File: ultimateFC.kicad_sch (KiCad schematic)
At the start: 205 parts, among them J1 USB_B_Micro, U1 LMR33630CQRNX, U2 TPS62824ADMQ, U3 LMR33620CRNXT, U4 S25FL064L, U5 DPS310, U6 BMI270, U7 STM32H735VGH6, U8 ICM-20602, Y1 CSTNE8M00G550000R0

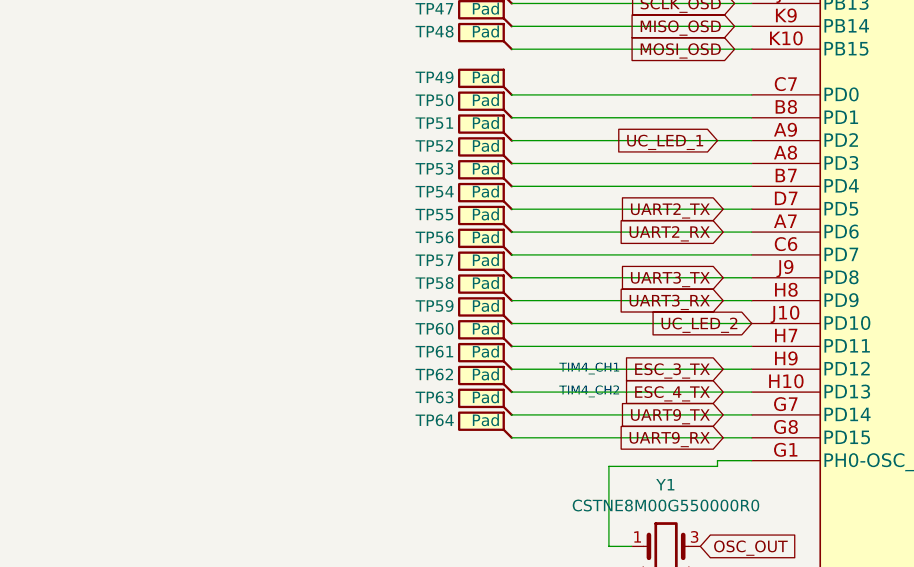
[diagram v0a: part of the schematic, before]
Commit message: more layout
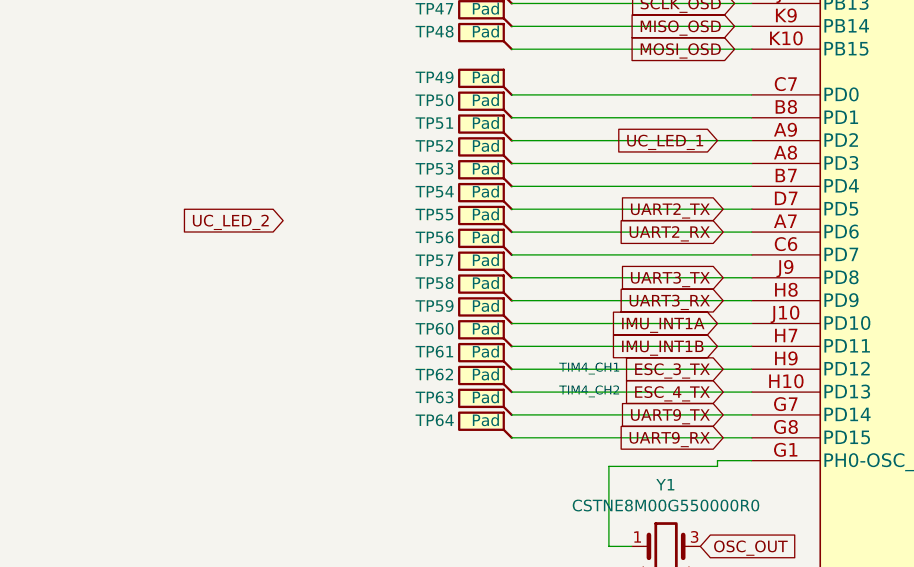
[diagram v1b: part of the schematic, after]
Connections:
- net UC_LED_2: no longer TP59.1, U7.J10 (PD10)
- net IMU_INT1B: now reaches TP60.1, U7.H7 (PD11)
- new net IMU_INT1A: TP59.1, U7.J10 (PD10)
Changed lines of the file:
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@@
+    )
+  )
+  (global_label "IMU_INT1A" (shape input) (at 538.48 127 180) (fields_autoplaced)
+    (effects (font (size 1.27 1.27)) (justify right))
+    (property "Intersheet References" "${INTERSHEET_REFS}" (id 0) (at 526.6006 126.9206 0)
+      (effects (font (size 1.27 1.27)) (justify right) hide)
     )
   )
@@
     )
   )
-  (global_label "UC_LED_2" (shape input) (at 542.29 127 180) (fields_autoplaced)
+  (global_label "UC_LED_2" (shape input) (at 490.22 115.57 180) (fields_autoplaced)
     (effects (font (size 1.27 1.27)) (justify right))
-    (property "Intersheet References" "${INTERSHEET_REFS}" (id 0) (at 0 0 0)
+    (property "Intersheet References" "${INTERSHEET_REFS}" (id 0) (at -52.07 -11.43 0)
       (effects (font (size 1.27 1.27)) hide)
     )
@@
     )
   )
+  (global_label "IMU_INT1B" (shape input) (at 538.48 129.54 180) (fields_autoplaced)
+    (effects (font (size 1.27 1.27)) (justify right))
+    (property "Intersheet References" "${INTERSHEET_REFS}" (id 0) (at 526.4191 129.4606 0)
+      (effects (font (size 1.27 1.27)) (justify right) hide)
+    )
+  )
